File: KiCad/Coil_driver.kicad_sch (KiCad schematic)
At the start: 44 parts, among them J1 USB_C_Receptacle_PowerOnly_6P, J2 Conn_01x07_Socket, J4 Conn_01x06_Socket, Q1 MMBT5551L, Q2 MMBT5551L, Q3 MMBT5551L, U1 MT3608, U2 PC817, U3 HIP4080A, U4 DMHT10H032LFJ, U5 MCP6002-xSN

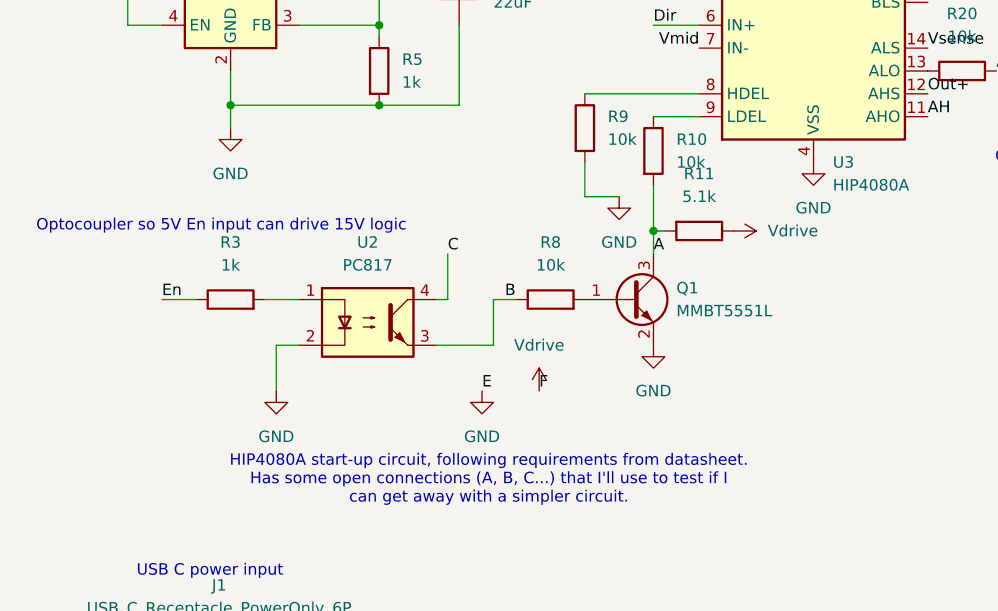
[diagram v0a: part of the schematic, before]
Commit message: schematic v1
lcsc, component values, and footprints not finalised. shit is too big rn.
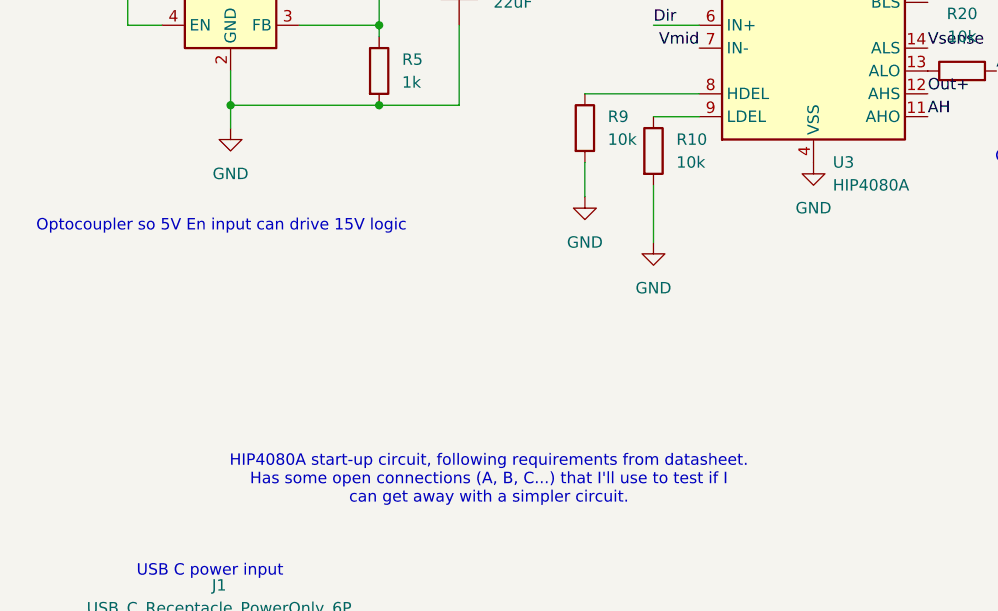
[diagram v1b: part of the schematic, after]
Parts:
- removed Q1: MMBT5551L, Package_TO_SOT_SMD:SOT-23, symbol Transistor_BJT:MMBT5551L
- removed R11: 5.1k, Resistor_SMD:R_0603_1608Metric, symbol Device:R
- removed R3: 1k, Resistor_SMD:R_0603_1608Metric, symbol Device:R
- removed R8: 10k, Resistor_SMD:R_0603_1608Metric, symbol Device:R
- removed U2: PC817, Package_DIP:DIP-4_W7.62mm, symbol Isolator:PC817
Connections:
- net A: no longer R10.2
- net GND: now also R10.2; no longer J4.4 (Pin_4)
- net Vdrive: no longer J4.5 (Pin_5)
- new net E: J4.4 (Pin_4)
- new net F: J4.5 (Pin_5)

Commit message: idk
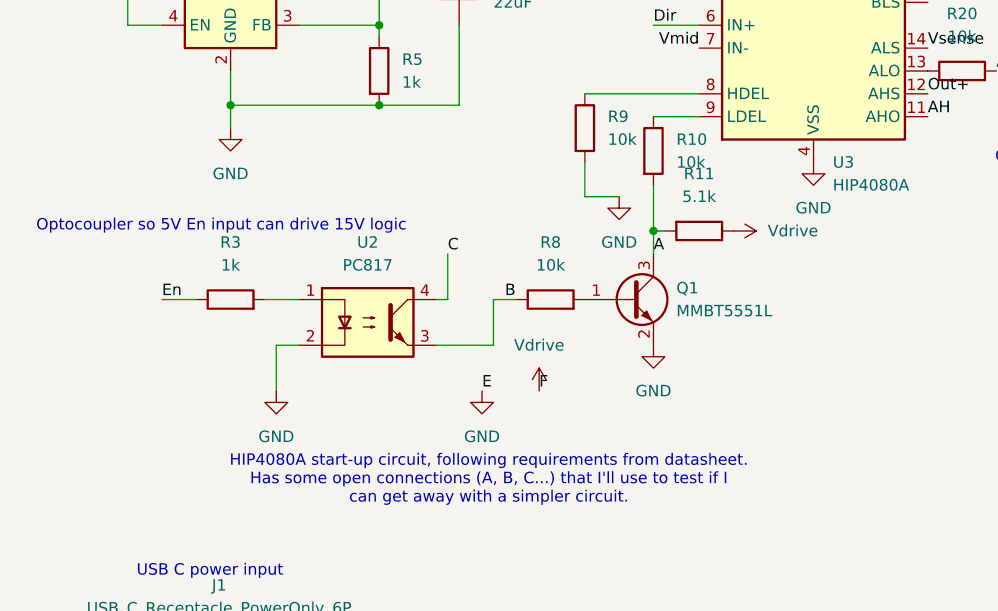
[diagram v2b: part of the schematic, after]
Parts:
- added Q1: MMBT5551L, Package_TO_SOT_SMD:SOT-23, symbol Transistor_BJT:MMBT5551L
- added R11: 5.1k, Resistor_SMD:R_0603_1608Metric, symbol Device:R
- added R3: 1k, Resistor_SMD:R_0603_1608Metric, symbol Device:R
- added R8: 10k, Resistor_SMD:R_0603_1608Metric, symbol Device:R
- added U2: PC817, Package_DIP:DIP-4_W7.62mm, symbol Isolator:PC817
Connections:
- net E is gone; now on net GND: J4.4 (Pin_4)
- net F is gone; now on net Vdrive: J4.5 (Pin_5)
- net A: now also R10.2, Q1.3 (C), R11.2
- net B: now also R8.1, U2.3
- net C: now also U2.4
- net En: now also R3.1
- net GND: now also Q1.2 (E), U2.2; no longer R10.2
- net Vdrive: now also R11.1
- new net: R3.2, U2.1
- new net: Q1.1 (B), R8.2
